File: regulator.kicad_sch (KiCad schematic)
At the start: 23 parts, among them U1 AMS1117-3.3

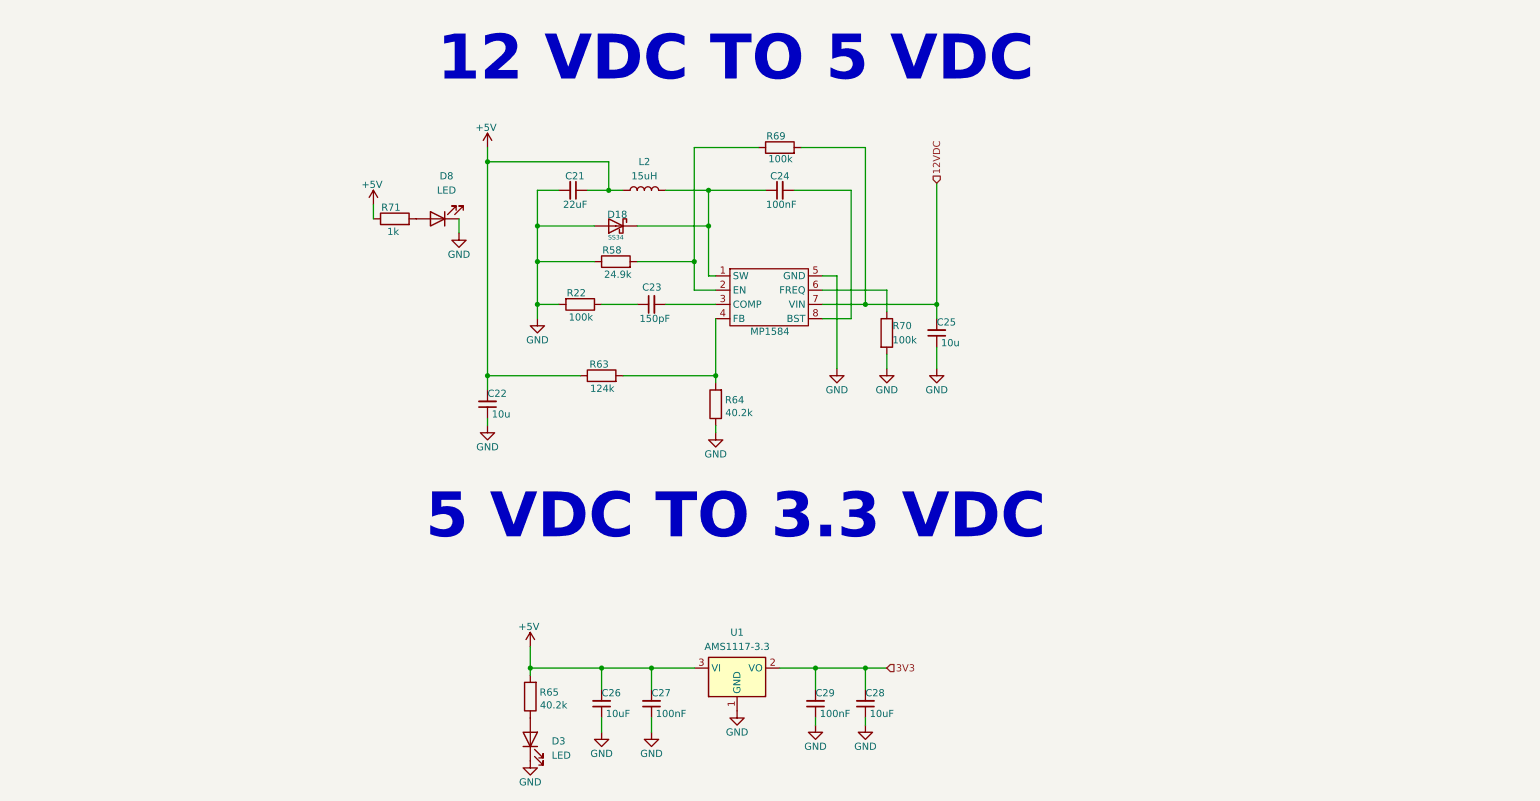
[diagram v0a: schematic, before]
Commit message: Schematic V1
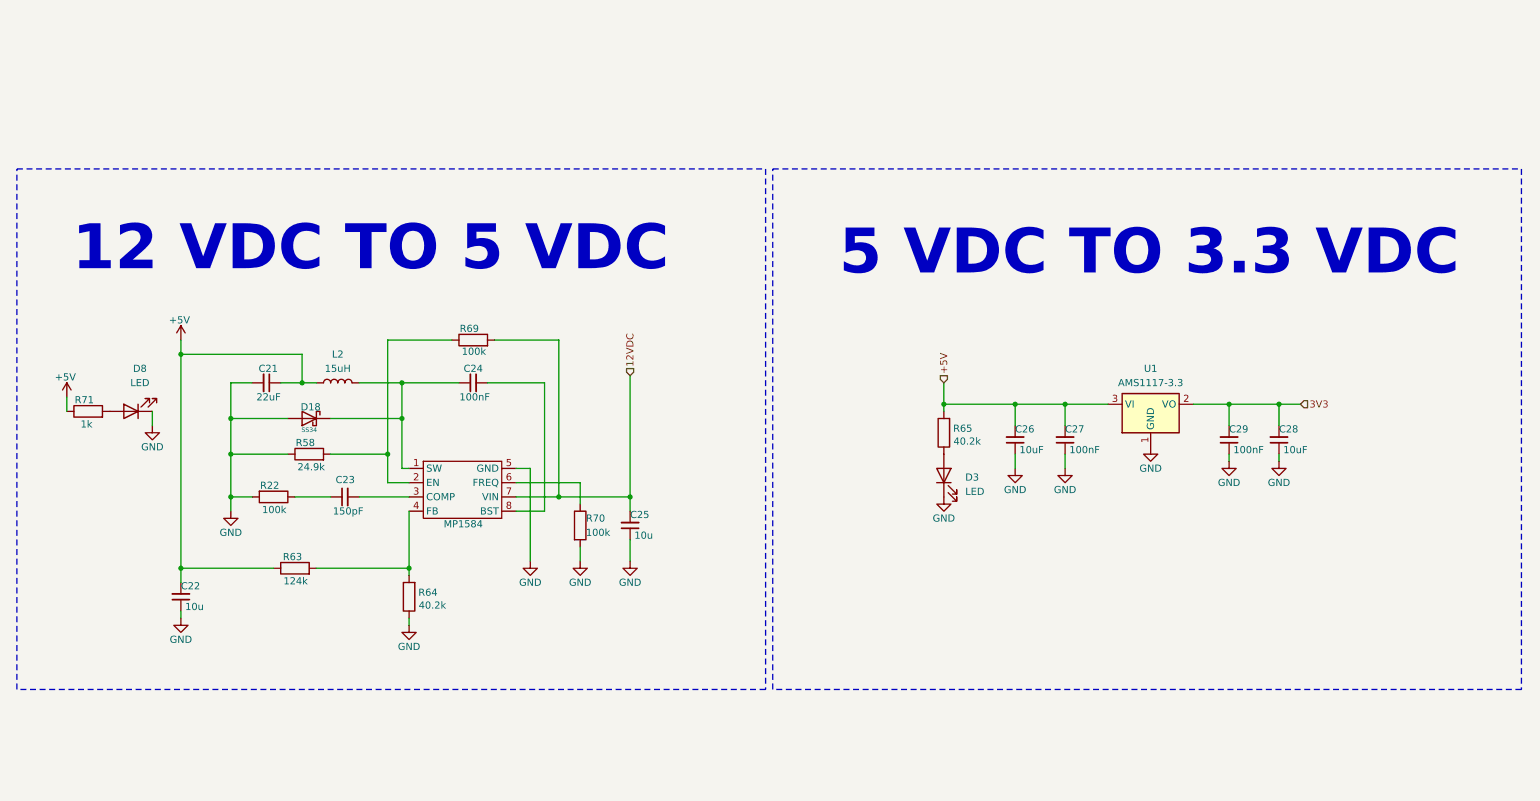
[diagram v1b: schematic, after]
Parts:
- D18: footprint PCM_JLCPCB:D_SMA -> Diode_SMD:D_SMA
- D3, D8: footprint (none) -> LED_SMD:LED_1206_3216Metric_Pad1.42x1.75mm_HandSolder
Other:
- title: Board Robot SUMO -> Board Robot SOCCER & SUMO
- moved on the sheet: C21, C22, C23, C24, C25, C26, C27, C28, C29, D18, D3, D8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

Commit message: layout v1.1
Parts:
- D3, D8: footprint LED_SMD:LED_1206_3216Metric_Pad1.42x1.75mm_HandSolder -> LED_SMD:LED_0805_2012Metric_Pad1.15x1.40mm_HandSolder
- MP1584: footprint Package_SO:SOIC-8-1EP_3.9x4.9mm_P1.27mm_EP2.41x3.81mm_ThermalVias -> Package_SO:SOIC-8-1EP_3.9x4.9mm_P1.27mm_EP2.29x3mm
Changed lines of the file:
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@@
 			)
 		)
-		(property "Footprint" "LED_SMD:LED_1206_3216Metric_Pad1.42x1.75mm_HandSolder"
+		(property "Footprint" "LED_SMD:LED_0805_2012Metric_Pad1.15x1.40mm_HandSolder"
 			(at 35.56 95.25 0)
 			(hide yes)
@@
 			)
 		)
-		(property "Footprint" "Package_SO:SOIC-8-1EP_3.9x4.9mm_P1.27mm_EP2.41x3.81mm_ThermalVias"
+		(property "Footprint" "Package_SO:SOIC-8-1EP_3.9x4.9mm_P1.27mm_EP2.29x3mm"
 			(at 94.996 115.57 0)
 			(hide yes)
@@
 			)
 		)
-		(property "Footprint" "LED_SMD:LED_1206_3216Metric_Pad1.42x1.75mm_HandSolder"
+		(property "Footprint" "LED_SMD:LED_0805_2012Metric_Pad1.15x1.40mm_HandSolder"
 			(at 180.34 106.68 0)
 			(hide yes)
